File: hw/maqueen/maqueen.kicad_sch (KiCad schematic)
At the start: 29 parts, among them IC1 MSP430FR2355TPT, J1 conn_DFrobot, J2 ESP01, SW1 RST, U1 LMV324

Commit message: constraints + crystal
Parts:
- removed C1, C4, C6, C8: 10u, symbol Device:C
- added Cload1, Cload2: 12.5n, Capacitor_SMD:C_0805_2012Metric, symbol Device:C
- added J3: SBW, Connector_PinHeader_2.54mm:PinHeader_1x03_P2.54mm_Vertical, symbol Connector_Generic:Conn_01x03
- added Y1: Crystal, Connector_PinHeader_1.27mm:PinHeader_1x02_P1.27mm_Vertical, symbol Device:Crystal
- C2, C3, C5, C7, C9: footprint (none) -> Capacitor_SMD:C_0805_2012Metric
- J2: footprint (none) -> Connector_PinHeader_2.54mm:PinHeader_2x04_P2.54mm_Vertical
- LCD1: footprint (none) -> MiSE:LCD_2x16_I2C(Midas)
- R10, R11, R5, R6, R7, R8, R9: footprint (none) -> Resistor_SMD:R_0805_2012Metric
- R2, R3: value 10k -> 2.2k; footprint (none) -> Resistor_SMD:R_0805_2012Metric
- S1: footprint THB001P -> MiSE:THB001P
- SW1: footprint (none) -> Button_Switch_THT:SW_PUSH_6mm
- U1: footprint (none) -> Package_SO:SOIC-14_3.9x8.7mm_P1.27mm
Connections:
- net GND: now also Cload1.2, Cload2.2, J3.3 (Pin_3)
- net TCK: now also J3.2 (Pin_2)
- net TDO/TDI: now also J3.1 (Pin_1)
- net at IC1.8 (P2.7/TB0CLK/XIN): now also Cload1.1, Y1.1
- net at IC1.9 (P2.6/MCLK/XOUT): now also Cload2.1, Y1.2
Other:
- note added: "DEBUG"
- moved on the sheet: C2, C3, C5, C7, C9, IC1, J1, J2, LCD1, R1, R10, R11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

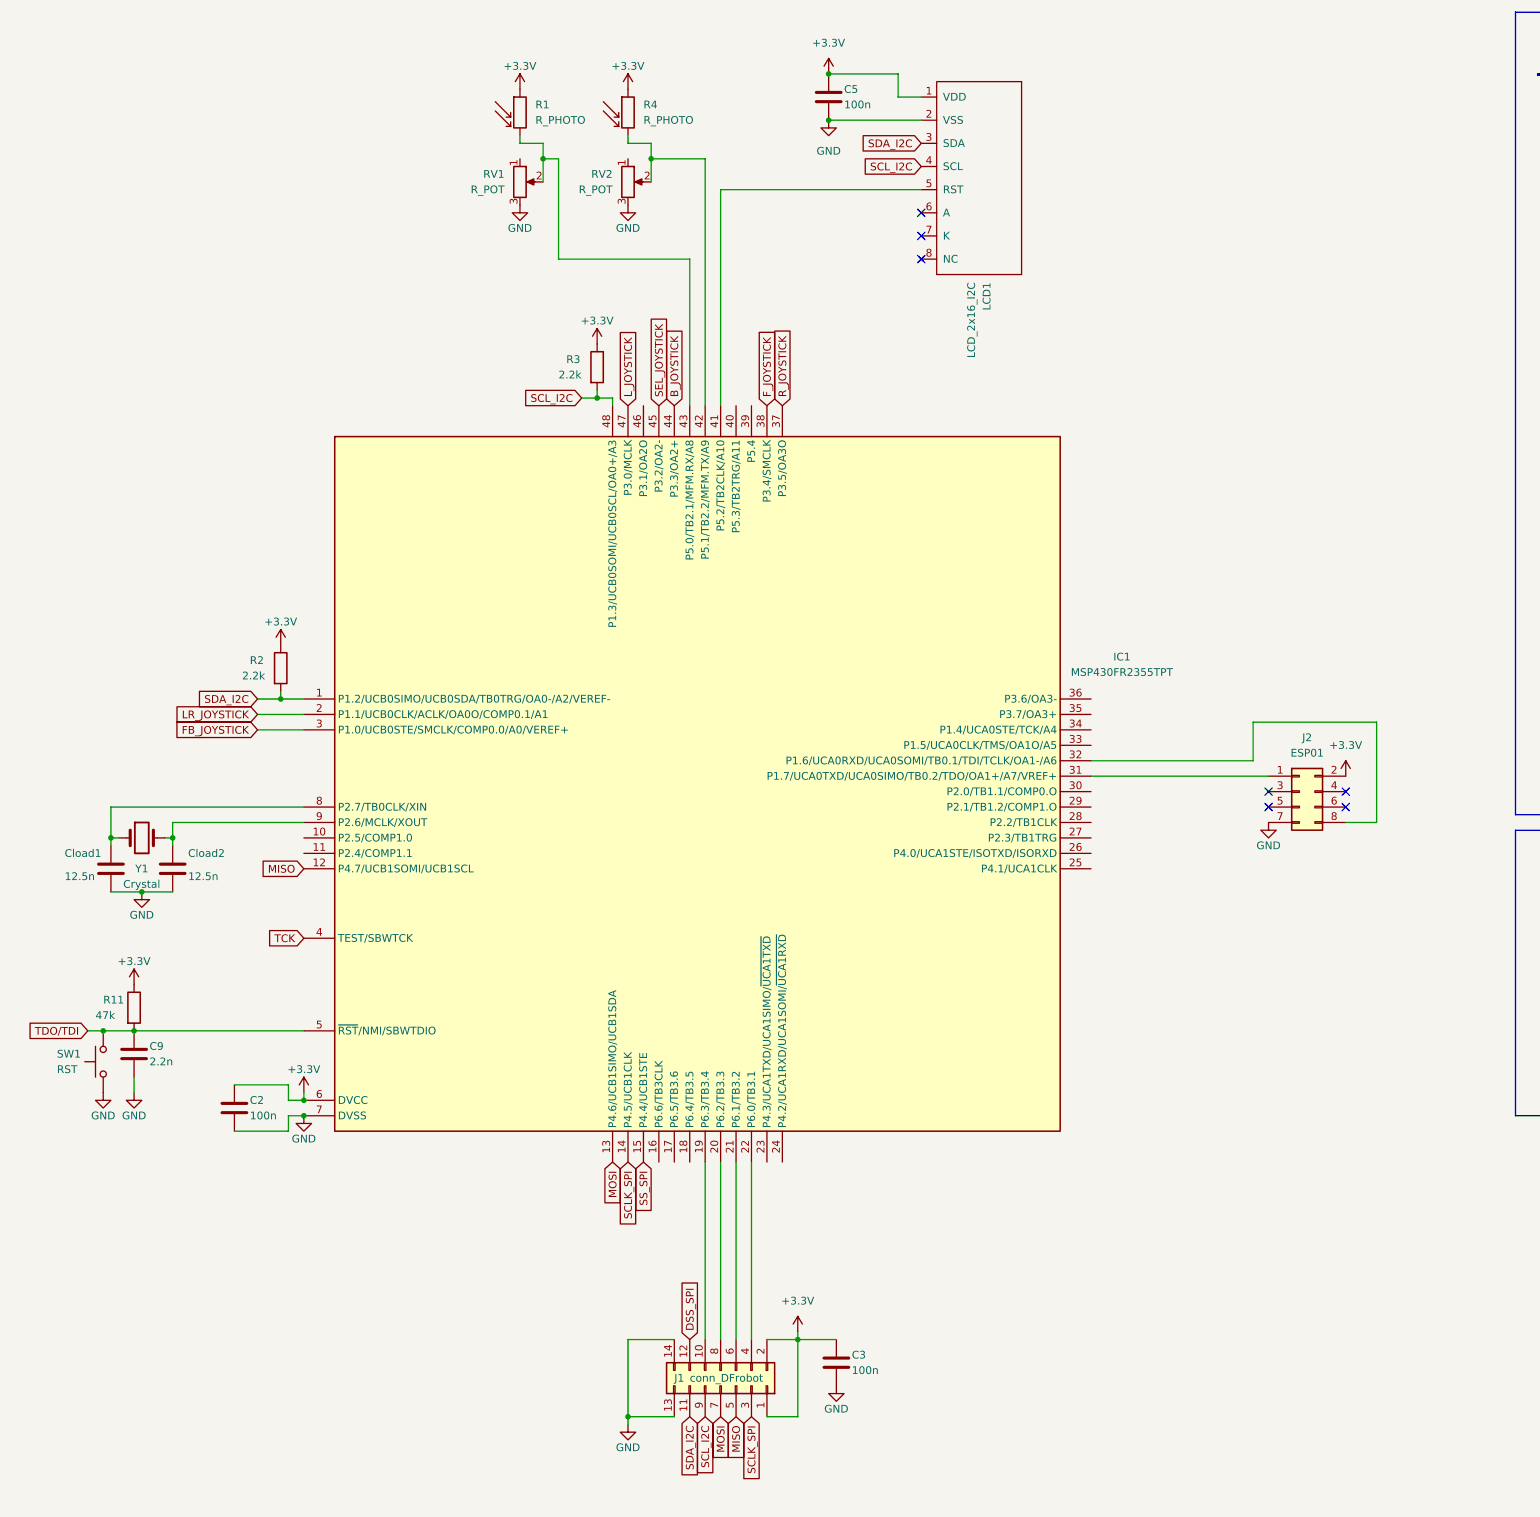
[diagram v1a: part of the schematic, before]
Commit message: netclasses, specs and more
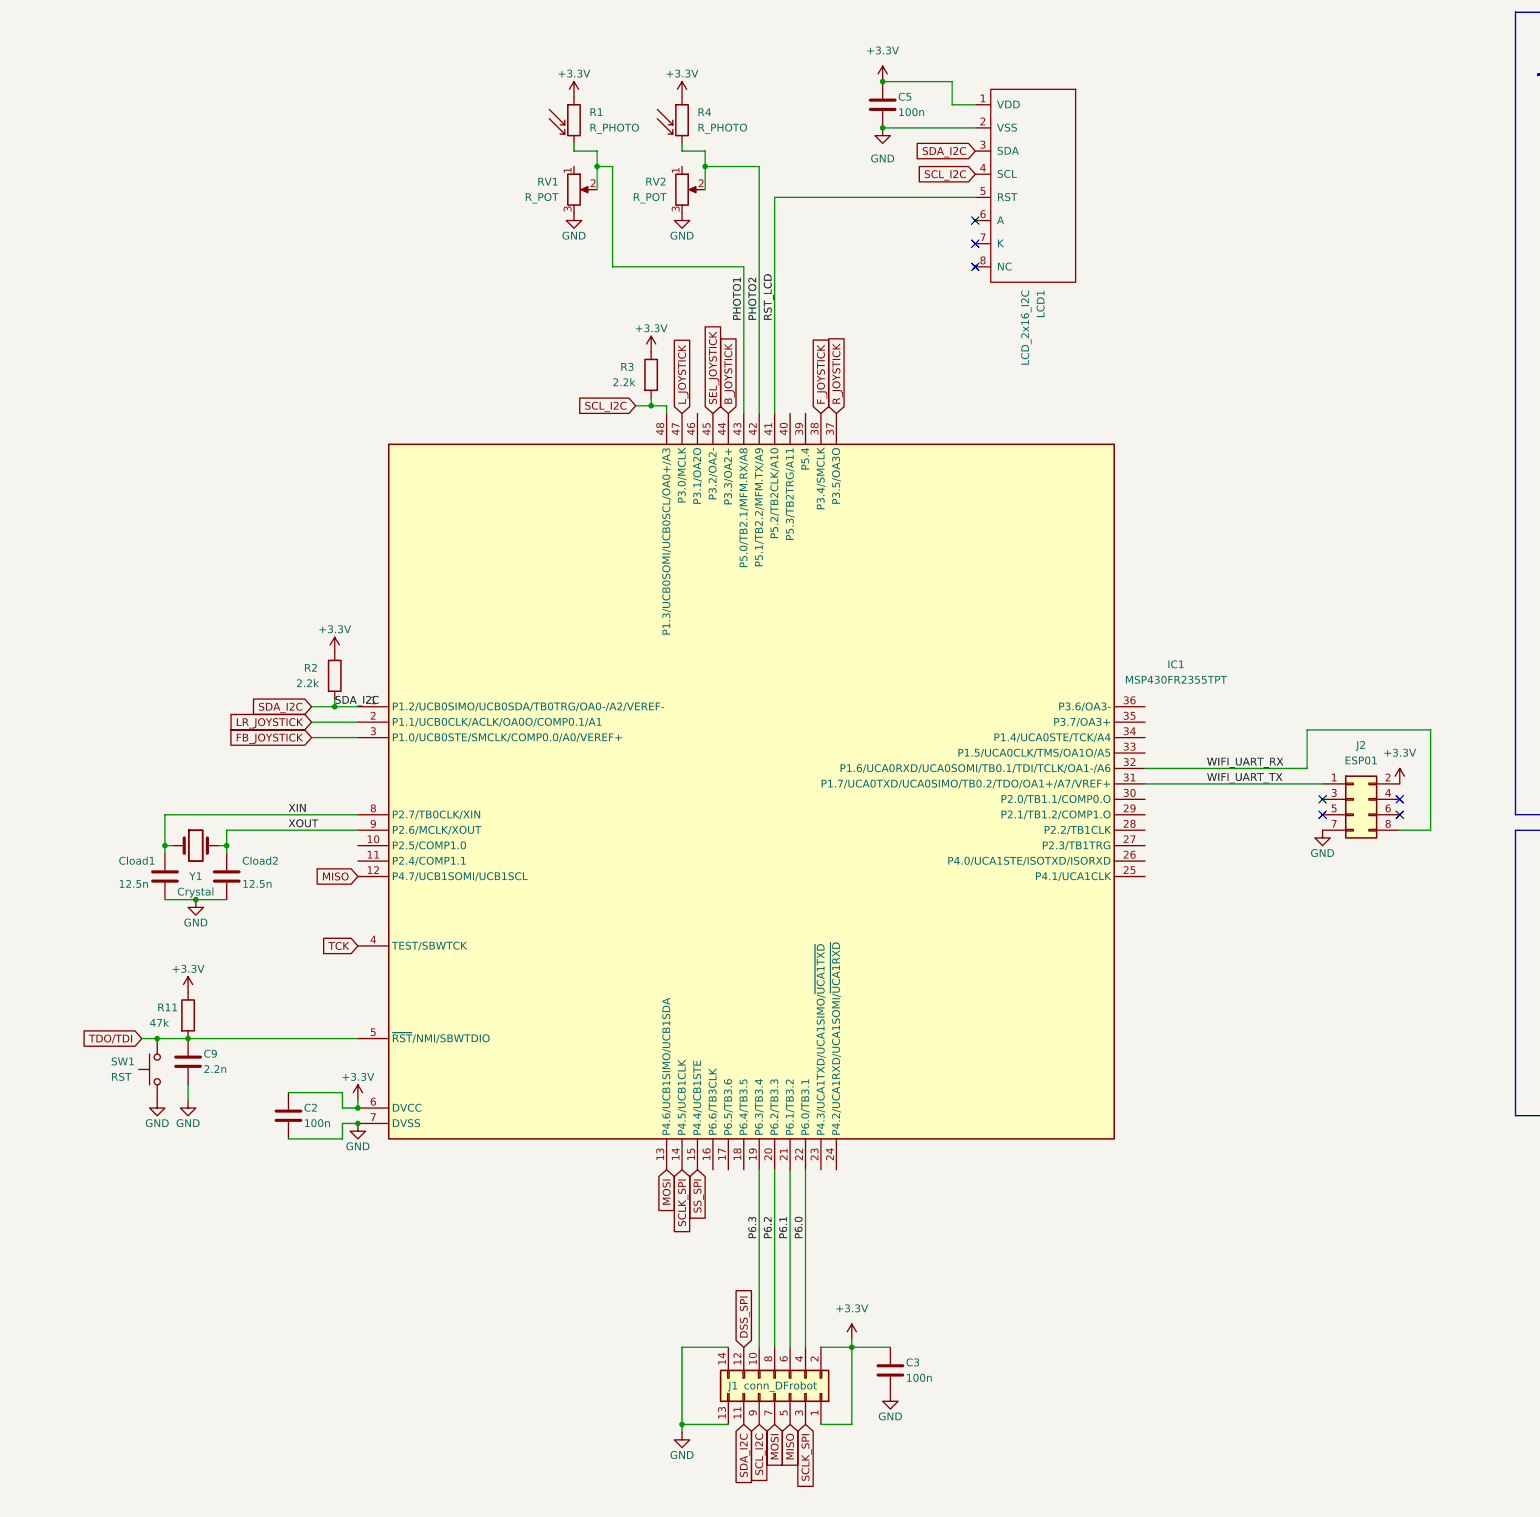
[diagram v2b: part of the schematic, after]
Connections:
- net PHOTO1: now reaches IC1.43 (P5.0/TB2.1/MFM.RX/A8), R1.2, RV1.2
- net XOUT: now reaches Cload2.1, IC1.9 (P2.6/MCLK/XOUT), Y1.2
- net XIN: now reaches Cload1.1, IC1.8 (P2.7/TB0CLK/XIN), Y1.1
- net WIFI_UART_TX: now reaches IC1.31 (P1.7/UCA0TXD/UCA0SIMO/TB0.2/TDO/OA1+/A7/VREF+), J2.1 (Pin_1)
- net WIFI_UART_RX: now reaches IC1.32 (P1.6/UCA0RXD/UCA0SOMI/TB0.1/TDI/TCLK/OA1-/A6), J2.8 (Pin_8)
- net PHOTO2: now reaches IC1.42 (P5.1/TB2.2/MFM.TX/A9), R4.2, RV2.2
- net P6.3: now reaches IC1.19 (P6.3/TB3.4), J1.10 (Pin_10)
- net P6.0: now reaches IC1.22 (P6.0/TB3.1), J1.4 (Pin_4)
- net P6.1: now reaches IC1.21 (P6.1/TB3.2), J1.6 (Pin_6)
- net P6.2: now reaches IC1.20 (P6.2/TB3.3), J1.8 (Pin_8)
- net RST_LCD: now reaches IC1.41 (P5.2/TB2CLK/A10), LCD1.5 (RST)
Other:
- moved on the sheet: C2, C3, C5, C9, Cload1, Cload2, IC1, J1, J2, LCD1, R1, R11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
